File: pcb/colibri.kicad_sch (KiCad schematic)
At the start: 92 parts

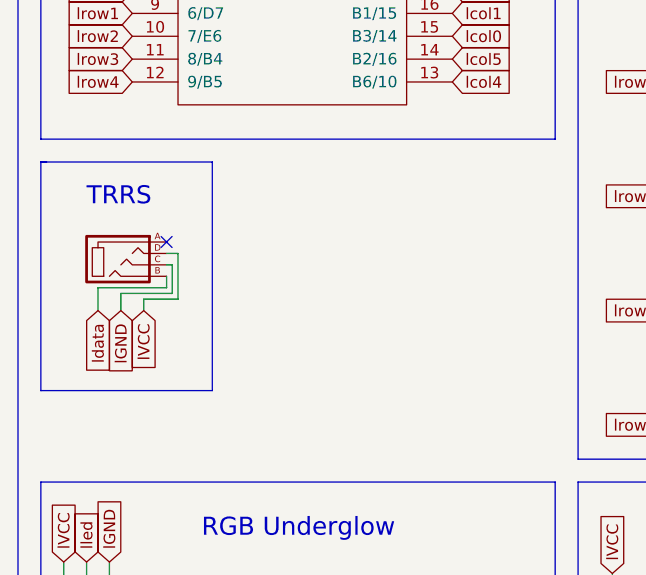
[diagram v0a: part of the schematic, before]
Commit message: reset button
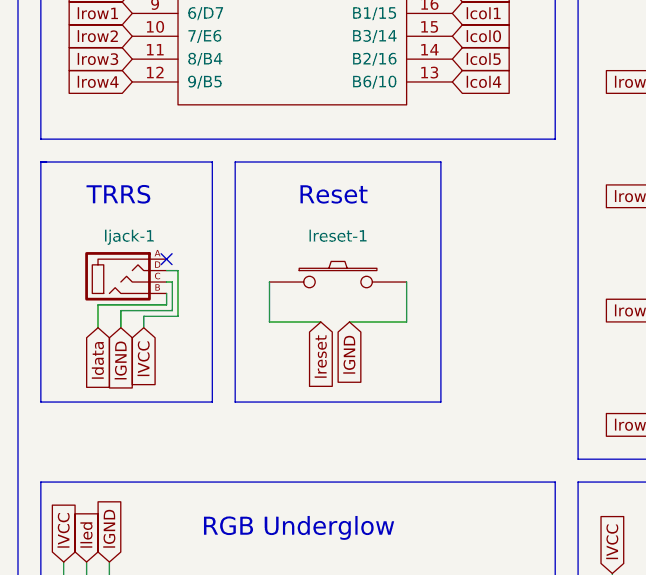
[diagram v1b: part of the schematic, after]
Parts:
- added lreset-1: SW_PUSH, kbd:ResetSW_4P, symbol kbd:SW_PUSH
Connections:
- net lGND: now also lreset-1.2
- net lreset: now also lreset-1.1
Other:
- note added: "Reset"
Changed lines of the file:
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@@
   (no_connect (at 35.56 54.61))
   (no_connect (at 71.12 54.61))
-  (no_connect (at 39.37 90.17))
+  (no_connect (at 39.37 92.075))
   (wire (pts (xy 163.83 78.74) (xy 163.83 91.44))
     (stroke (width 0) (type default) (color 0 0 0 0))
@@
     (stroke (width 0) (type default) (color 0 0 0 0))
   )
-  (wire (pts (xy 40.005 95.885) (xy 34.29 95.885))
+  (wire (pts (xy 40.005 97.79) (xy 34.29 97.79))
     (stroke (width 0) (type default) (color 0 0 0 0))
   )
@@
     (stroke (width 0) (type default) (color 0 0 0 0))
   )
-  (wire (pts (xy 40.64 91.44) (xy 40.64 96.52))
+  (wire (pts (xy 40.64 93.345) (xy 40.64 98.425))
     (stroke (width 0) (type default) (color 0 0 0 0))
   )
@@
     (stroke (width 0) (type default) (color 0 0 0 0))
   )
-  (polyline (pts (xy 44.45 106.68) (xy 25.4 106.68))
+  (polyline (pts (xy 44.45 107.95) (xy 25.4 107.95))
     (stroke (width 0) (type solid) (color 0 0 0 0))
   )
@@
     (stroke (width 0) (type solid) (color 0 0 0 0))
   )
-  (wire (pts (xy 40.64 96.52) (xy 36.83 96.52))
+  (wire (pts (xy 40.64 98.425) (xy 36.83 98.425))
     (stroke (width 0) (type default) (color 0 0 0 0))
   )
@@
     (stroke (width 0) (type default) (color 0 0 0 0))
   )
+  (polyline (pts (xy 69.85 107.95) (xy 46.99 107.95))
+    (stroke (width 0) (type solid) (color 0 0 0 0))
+  )
   (wire (pts (xy 176.53 134.62) (xy 177.8 134.62))
     (stroke (width 0) (type default) (color 0 0 0 0))
@@
     (stroke (width 0) (type default) (color 0 0 0 0))
   )
-  (wire (pts (xy 39.37 93.98) (xy 39.37 95.25))
+  (wire (pts (xy 39.37 95.885) (xy 39.37 97.155))
     (stroke (width 0) (type default) (color 0 0 0 0))
   )
@@
     (stroke (width 0) (type default) (color 0 0 0 0))
   )
-  (polyline (pts (xy 44.45 81.28) (xy 44.45 106.68))
+  (polyline (pts (xy 44.45 81.28) (xy 44.45 107.95))
     (stroke (width 0) (type solid) (color 0 0 0 0))
   )
@@
     (stroke (width 0) (type default) (color 0 0 0 0))
   )
+  (polyline (pts (xy 46.99 81.28) (xy 69.85 81.28))
+    (stroke (width 0) (type solid) (color 0 0 0 0))
+  )
   (wire (pts (xy 124.46 195.58) (xy 125.73 195.58))
     (stroke (width 0) (type default) (color 0 0 0 0))
@@
     (stroke (width 0) (type default) (color 0 0 0 0))
   )
+  (polyline (pts (xy 46.99 107.95) (xy 46.99 81.28))
+    (stroke (width 0) (type solid) (color 0 0 0 0))
+  )
+  (wire (pts (xy 66.04 99.06) (xy 66.04 94.615))
+    (stroke (width 0) (type default) (color 0 0 0 0))
+  )
   (wire (pts (xy 162.56 66.04) (xy 162.56 68.58))
     (stroke (width 0) (type default) (color 0 0 0 0))
@@
     (stroke (width 0) (type solid) (color 0 0 0 0))
   )
-  (polyline (pts (xy 25.4 106.68) (xy 25.4 81.28))
+  (polyline (pts (xy 25.4 107.95) (xy 25.4 81.28))
     (stroke (width 0) (type solid) (color 0 0 0 0))
   )
@@
     (stroke (width 0) (type default) (color 0 0 0 0))
   )
+  (wire (pts (xy 56.515 99.06) (xy 50.8 99.06))
+    (stroke (width 0) (type default) (color 0 0 0 0))
+  )
   (wire (pts (xy 171.45 85.09) (xy 187.96 85.09))
     (stroke (width 0) (type default) (color 0 0 0 0))
@@
     (stroke (width 0) (type default) (color 0 0 0 0))
   )
-  (wire (pts (xy 34.29 95.885) (xy 34.29 97.79))
+  (wire (pts (xy 34.29 97.79) (xy 34.29 99.695))
     (stroke (width 0) (type default) (color 0 0 0 0))
   )
@@
     (stroke (width 0) (type default) (color 0 0 0 0))
   )
-  (wire (pts (xy 39.37 91.44) (xy 40.64 91.44))
+  (wire (pts (xy 39.37 93.345) (xy 40.64 93.345))
     (stroke (width 0) (type default) (color 0 0 0 0))
   )
@@
     (stroke (width 0) (type default) (color 0 0 0 0))
   )
-  (wire (pts (xy 40.005 92.71) (xy 40.005 95.885))
+  (wire (pts (xy 40.005 94.615) (xy 40.005 97.79))
     (stroke (width 0) (type default) (color 0 0 0 0))
   )
@@
     (stroke (width 0) (type default) (color 0 0 0 0))
   )
-  (wire (pts (xy 31.75 95.25) (xy 31.75 97.79))
+  (wire (pts (xy 31.75 97.155) (xy 31.75 99.695))
     (stroke (width 0) (type default) (color 0 0 0 0))
   )
@@
     (stroke (width 0) (type default) (color 0 0 0 0))
   )
-  (wire (pts (xy 39.37 95.25) (xy 31.75 95.25))
+  (wire (pts (xy 39.37 97.155) (xy 31.75 97.155))
+    (stroke (width 0) (type default) (color 0 0 0 0))
+  )
+  (wire (pts (xy 59.69 99.06) (xy 66.04 99.06))
     (stroke (width 0) (type default) (color 0 0 0 0))
   )
@@
     (stroke (width 0) (type default) (color 0 0 0 0))
   )
-  (wire (pts (xy 39.37 92.71) (xy 40.005 92.71))
+  (wire (pts (xy 39.37 94.615) (xy 40.005 94.615))
     (stroke (width 0) (type default) (color 0 0 0 0))
   )
@@
     (stroke (width 0) (type default) (color 0 0 0 0))
   )
-  (wire (pts (xy 36.83 96.52) (xy 36.83 97.79))
+  (wire (pts (xy 36.83 98.425) (xy 36.83 99.695))
     (stroke (width 0) (type default) (color 0 0 0 0))
   )
@@
   (wire (pts (xy 124.46 165.1) (xy 125.73 165.1))
     (stroke (width 0) (type default) (color 0 0 0 0))
+  )
+  (wire (pts (xy 50.8 99.06) (xy 50.8 94.615))
+    (stroke (width 0) (type default) (color 0 0 0 0))
+  )
+  (polyline (pts (xy 69.85 81.28) (xy 69.85 107.95))
+    (stroke (width 0) (type solid) (color 0 0 0 0))
   )
   (wire (pts (xy 69.85 143.51) (xy 69.85 144.78))
@@
   (text "RGB Underglow" (at 64.77 123.19 180)
     (effects (font (size 2 2)) (justify right bottom))
+  )
+  (text "Reset" (at 53.975 86.36 0)
+    (effects (font (size 2 2)) (justify left bottom))
   )
   (global_label "lcol3" (shape input) (at 71.12 59.69 0) (fields_autoplaced)
@@
     )
   )
-  (global_label "lVCC" (shape input) (at 36.83 97.79 270) (fields_autoplaced)
+  (global_label "lVCC" (shape input) (at 36.83 99.695 270) (fields_autoplaced)
     (effects (font (size 1.27 1.27)) (justify right))
-    (property "Intersheet References" "${INTERSHEET_REFS}" (id 0) (at 36.9094 104.4969 90)
+    (property "Intersheet References" "${INTERSHEET_REFS}" (id 0) (at 36.9094 106.4019 90)
       (effects (font (size 1.27 1.27)) (justify right) hide)
     )
@@
     )
   )
-  (global_label "ldata" (shape input) (at 31.75 97.79 270) (fields_autoplaced)
+  (global_label "ldata" (shape input) (at 31.75 99.695 270) (fields_autoplaced)
     (effects (font (size 1.27 1.27)) (justify right))
-    (property "Intersheet References" "${INTERSHEET_REFS}" (id 0) (at 31.6706 105.0412 90)
+    (property "Intersheet References" "${INTERSHEET_REFS}" (id 0) (at 31.6706 106.9462 90)
       (effects (font (size 1.27 1.27)) (justify right) hide)
     )
@@
     )
   )
+  (global_label "lGND" (shape input) (at 59.69 99.06 270) (fields_autoplaced)
+    (effects (font (size 1.27 1.27)) (justify right))
+    (property "Intersheet References" "${INTERSHEET_REFS}" (id 0) (at 59.7694 106.0088 90)
+      (effects (font (size 1.27 1.27)) (justify right) hide)
+    )
+  )
   (global_label "ldata" (shape input) (at 35.56 46.99 180) (fields_autoplaced)
     (effects (font (size 1.27 1.27)) (justify right))
@@
     )
   )
-  (global_label "lGND" (shape input) (at 34.29 97.79 270) (fields_autoplaced)
+  (global_label "lGND" (shape input) (at 34.29 99.695 270) (fields_autoplaced)
     (effects (font (size 1.27 1.27)) (justify right))
-    (property "Intersheet References" "${INTERSHEET_REFS}" (id 0) (at 34.2106 104.7388 90)
+    (property "Intersheet References" "${INTERSHEET_REFS}" (id 0) (at 34.2106 106.6438 90)
+      (effects (font (size 1.27 1.27)) (justify right) hide)
+    )
+  )
+  (global_label "lreset" (shape input) (at 56.515 99.06 270) (fields_autoplaced)
+    (effects (font (size 1.27 1.27)) (justify right))
+    (property "Intersheet References" "${INTERSHEET_REFS}" (id 0) (at 56.5944 106.8555 90)
       (effects (font (size 1.27 1.27)) (justify right) hide)
     )
@@
     (pin "2")
   )
-  (symbol (lib_id "kbd:MJ-4PP-9") (at 34.29 92.075 0) (unit 1)
-    (in_bom yes) (on_board yes)
-    (property "Reference" "ljack-1" (id 0) (at 38.1 87.63 0)
-      (effects (font (size 1.27 1.27)) (justify right) hide)
-    )
-    (property "Value" "MJ-4PP-9" (id 1) (at 33.9725 86.995 0)
-      (effects (font (size 1.27 1.27)) hide)
-    )
-    (property "Footprint" "kbd:MJ-4PP-9_1side" (id 2) (at 41.275 87.63 0)
-      (effects (font (size 1.27 1.27)) hide)
-    )
-    (property "Datasheet" "~" (id 3) (at 41.275 87.63 0)
+  (symbol (lib_id "kbd:MJ-4PP-9") (at 34.29 93.98 0) (unit 1)
+    (in_bom yes) (on_board yes)
+    (property "Reference" "ljack-1" (id 0) (at 38.1 89.535 0)
+      (effects (font (size 1.27 1.27)) (justify right))
+    )
+    (property "Value" "MJ-4PP-9" (id 1) (at 33.9725 88.9 0)
+      (effects (font (size 1.27 1.27)) hide)
+    )
+    (property "Footprint" "kbd:MJ-4PP-9_1side" (id 2) (at 41.275 89.535 0)
+      (effects (font (size 1.27 1.27)) hide)
+    )
+    (property "Datasheet" "~" (id 3) (at 41.275 89.535 0)
       (effects (font (size 1.27 1.27)) hide)
     )
@@
     (pin "3")
     (pin "4")
+  )
+  (symbol (lib_id "kbd:SW_PUSH") (at 58.42 94.615 0) (unit 1)
+    (in_bom yes) (on_board yes) (fields_autoplaced)
+    (property "Reference" "lreset-1" (id 0) (at 58.42 89.535 0))
+    (property "Value" "SW_PUSH" (id 1) (at 58.42 89.535 0)
+      (effects (font (size 1.27 1.27)) hide)
+    )
+    (property "Footprint" "kbd:ResetSW_4P" (id 2) (at 58.42 94.615 0)
+      (effects (font (size 1.27 1.27)) hide)
+    )
+    (property "Datasheet" "" (id 3) (at 58.42 94.615 0))
+    (pin "1")
+    (pin "2")
   )
   (symbol (lib_id "kbd:YS-SK6812MINI-E") (at 133.35 165.1 90) (unit 1)
@@
       (reference "lled-28") (unit 1) (value "YS-SK6812MINI-E") (footprint "kbd:YS-SK6812MINI-E")
     )
+    (path "/f45bfb45-f489-4e83-ba10-e93859f41fe6"
+      (reference "lreset-1") (unit 1) (value "SW_PUSH") (footprint "kbd:ResetSW_4P")
+    )
     (path "/377a23d8-2fa5-459f-9dad-5a649e830e53"
